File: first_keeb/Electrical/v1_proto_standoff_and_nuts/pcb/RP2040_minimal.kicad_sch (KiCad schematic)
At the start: 75 parts, among them J1 Conn_01x04_Socket, P1 USB-TYPE-C-016, Q1 SN74LV1T34DBV, SW1 SK-3296S-01-L3, SW2 MS-22C01-G010, SW3 TS-1187A-B-A-B, SW4 MS-22C01-G010, SW5 TS-1187A-B-A-B, SW6 BUTT1, SW7 BUTT3, SW8 BUTT2, U1 ME6206A25XG, U2 ME6208A44M3G, U3 PRTR5V0U2X, U4 MCP6001-OT, U5 STM32F401RCTx, U6 MCP6001-OT, U7 SLSS49E, U8 SLSS49E, U9 SLSS49E, Y1 8MHz

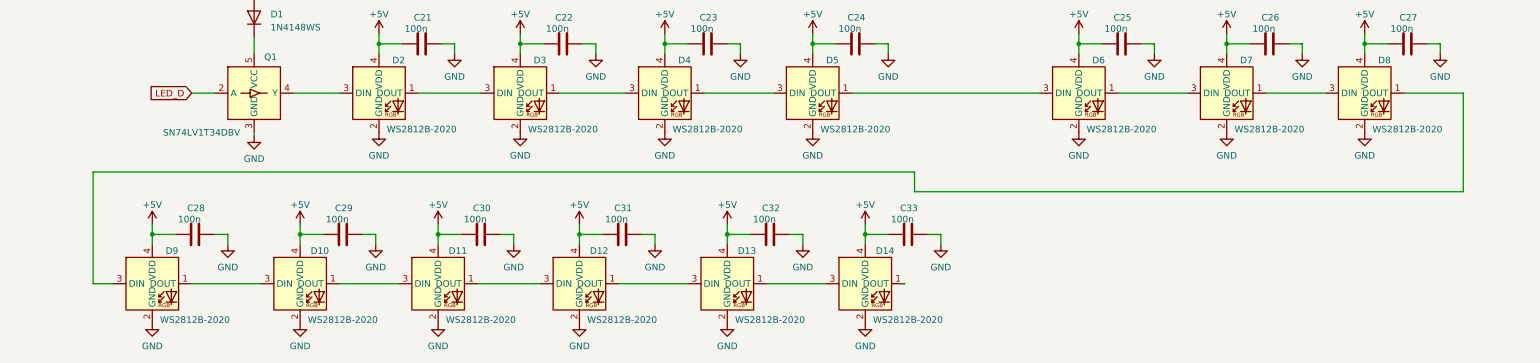
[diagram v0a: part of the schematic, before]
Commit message: add svg
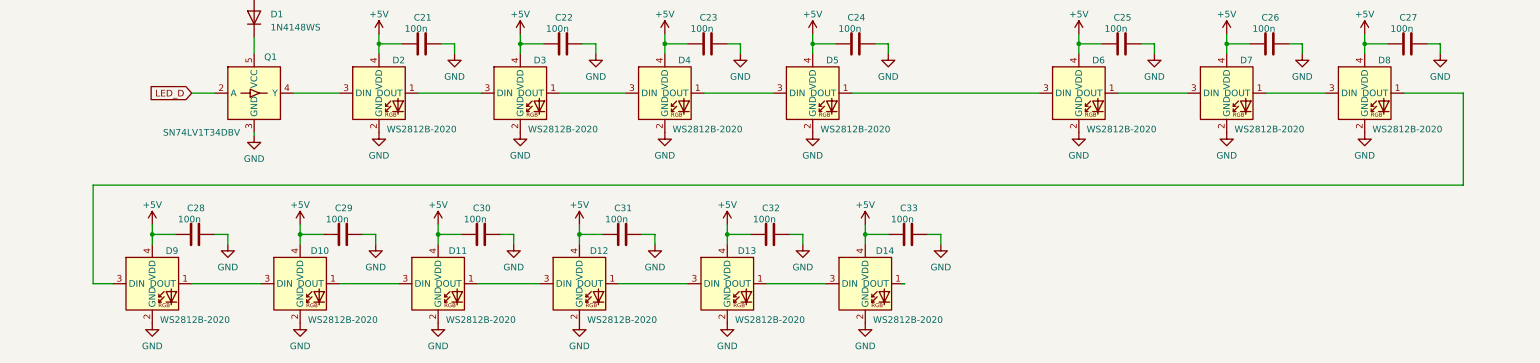
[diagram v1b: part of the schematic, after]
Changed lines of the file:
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@@
-    (stroke (width 0) (type default))
-  )
-  (wire (pts (xy 393.7 245.11) (xy 287.655 245.11))
     (stroke (width 0) (type default))
   )
@@
     (stroke (width 0) (type default))
   )
-  (wire (pts (xy 393.7 226.06) (xy 393.7 245.11))
+  (wire (pts (xy 393.7 226.06) (xy 393.7 243.84))
     (stroke (width 0) (type default))
   )
@@
     (stroke (width 0) (type default))
   )
-  (wire (pts (xy 287.655 241.3) (xy 287.655 245.11))
-    (stroke (width 0) (type default))
-  )
   (wire (pts (xy 313.69 92.71) (xy 314.96 92.71))
     (stroke (width 0) (type default))
@@
     (stroke (width 0) (type default))
   )
-  (wire (pts (xy 128.905 241.3) (xy 128.905 262.89))
+  (wire (pts (xy 128.905 243.84) (xy 128.905 262.89))
     (stroke (width 0) (type default))
   )
@@
     (stroke (width 0) (type default))
   )
-  (wire (pts (xy 128.905 241.3) (xy 287.655 241.3))
-    (stroke (width 0) (type default))
-  )
+  (wire (pts (xy 128.905 243.84) (xy 393.7 243.84))
+    (stroke (width 0) (type default))
+  )
